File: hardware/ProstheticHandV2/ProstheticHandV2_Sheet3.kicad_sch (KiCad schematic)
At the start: 0 parts

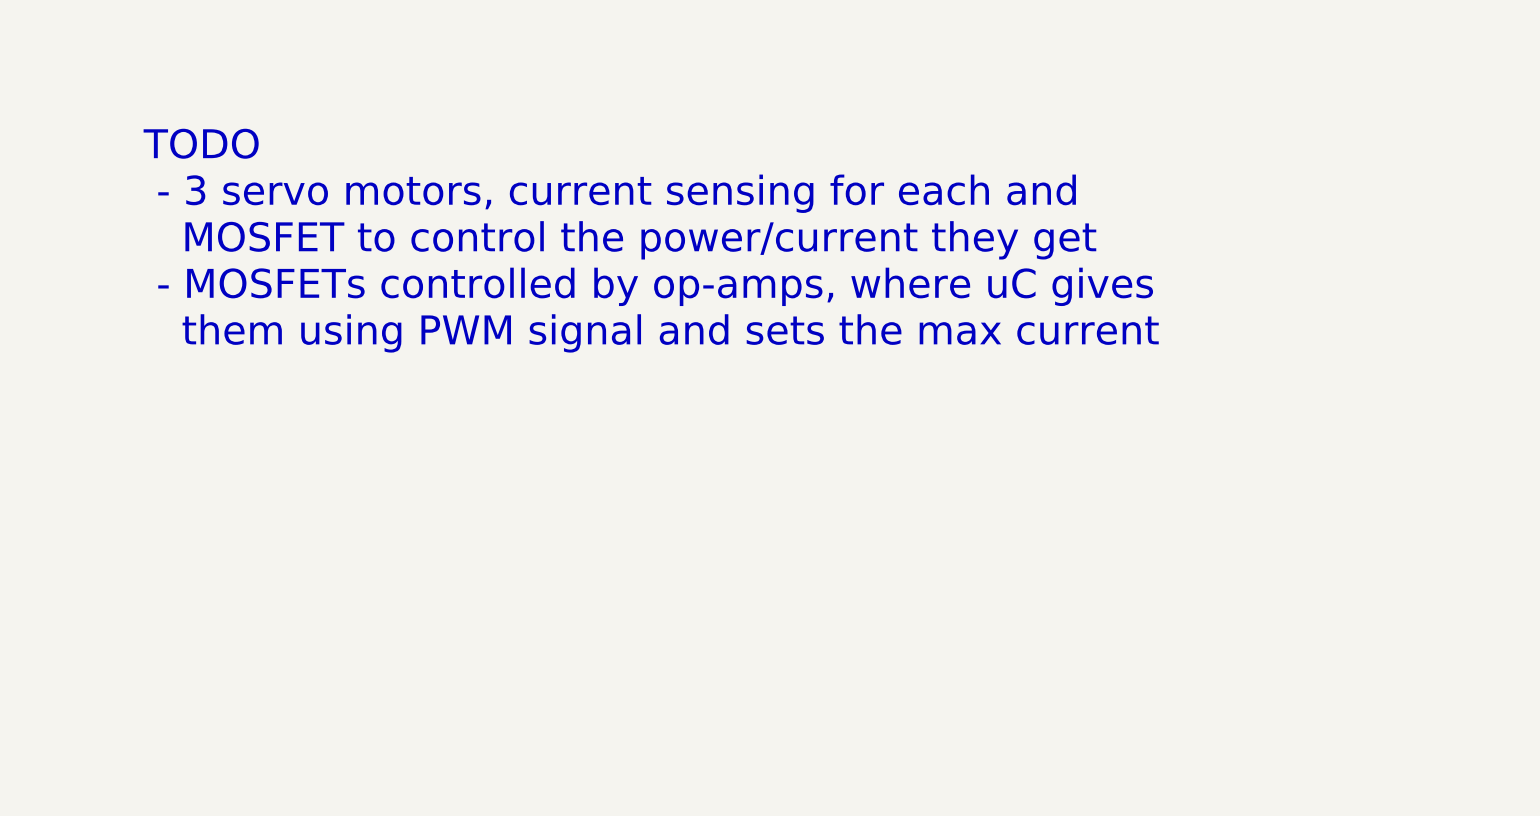
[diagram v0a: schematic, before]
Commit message: Started working on PCB
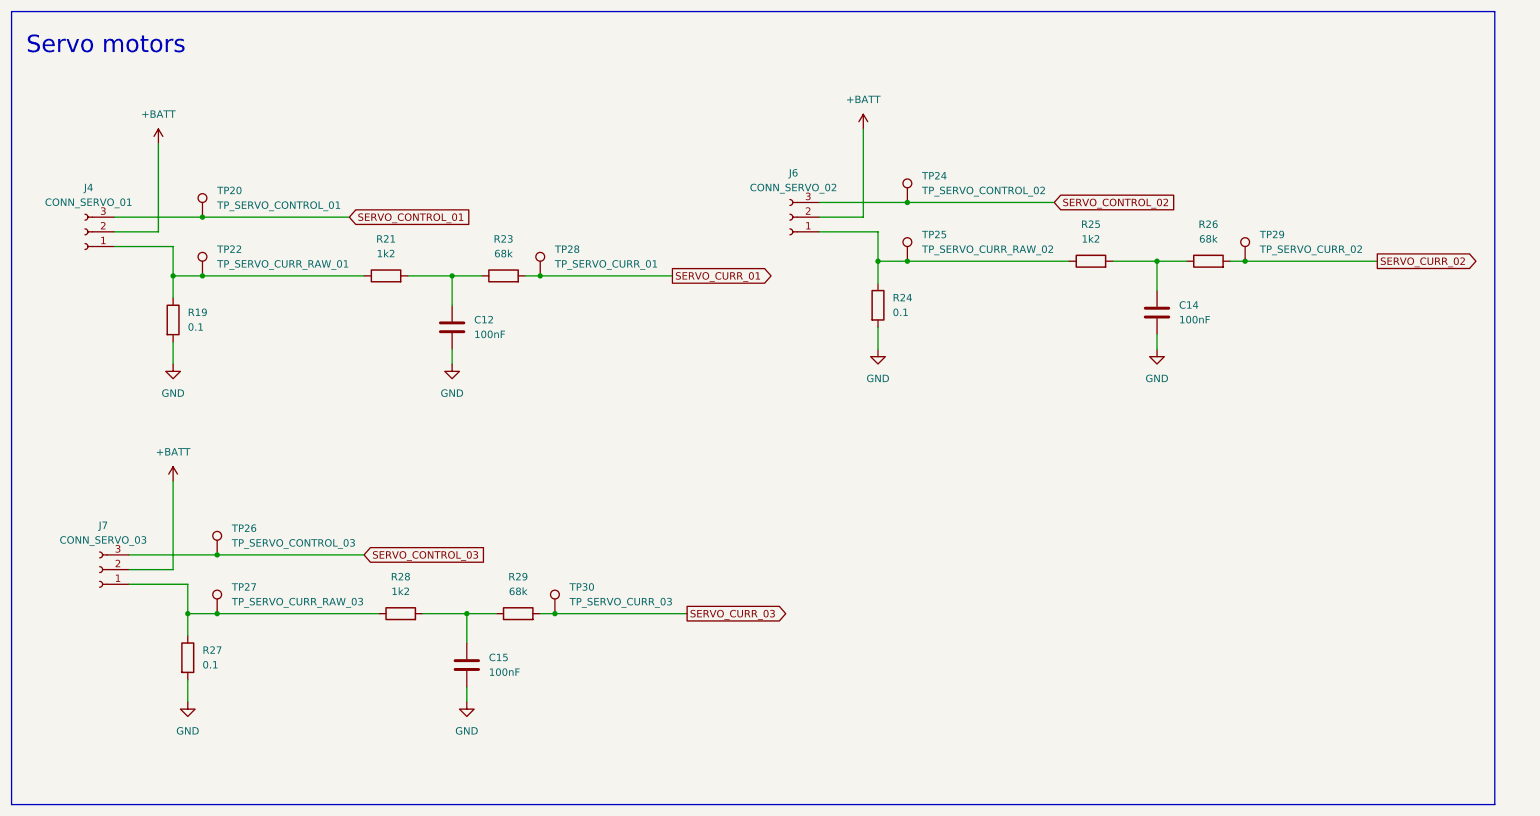
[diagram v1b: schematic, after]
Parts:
- added C12, C14, C15: 100nF, Capacitor_THT:C_Disc_D3.8mm_W2.6mm_P2.50mm, symbol Device:C
- added J4: CONN_SERVO_01, Connector_JST:JST_XA_B03B-XASK-1_1x03_P2.50mm_Vertical, symbol Connector:Conn_01x03_Socket
- added J6: CONN_SERVO_02, Connector_JST:JST_XA_B03B-XASK-1_1x03_P2.50mm_Vertical, symbol Connector:Conn_01x03_Socket
- added J7: CONN_SERVO_03, Connector_JST:JST_XA_B03B-XASK-1_1x03_P2.50mm_Vertical, symbol Connector:Conn_01x03_Socket
- added R19, R24, R27: 0.1, Resistor_THT:R_Axial_DIN0922_L20.0mm_D9.0mm_P30.48mm_Horizontal, symbol Device:R
- added R21, R25, R28: 1k2, Resistor_THT:R_Axial_DIN0207_L6.3mm_D2.5mm_P7.62mm_Horizontal, symbol Device:R
- added R23, R26, R29: 68k, Resistor_THT:R_Axial_DIN0207_L6.3mm_D2.5mm_P7.62mm_Horizontal, symbol Device:R
- added TP20: TP_SERVO_CONTROL_01, TestPoint:TestPoint_Pad_D2.5mm, symbol Connector:TestPoint
- added TP22: TP_SERVO_CURR_RAW_01, TestPoint:TestPoint_Pad_D2.5mm, symbol Connector:TestPoint
- added TP24: TP_SERVO_CONTROL_02, TestPoint:TestPoint_Pad_D2.5mm, symbol Connector:TestPoint
- added TP25: TP_SERVO_CURR_RAW_02, TestPoint:TestPoint_Pad_D2.5mm, symbol Connector:TestPoint
- added TP26: TP_SERVO_CONTROL_03, TestPoint:TestPoint_Pad_D2.5mm, symbol Connector:TestPoint
- added TP27: TP_SERVO_CURR_RAW_03, TestPoint:TestPoint_Pad_D2.5mm, symbol Connector:TestPoint
- added TP28: TP_SERVO_CURR_01, TestPoint:TestPoint_Pad_D2.5mm, symbol Connector:TestPoint
- added TP29: TP_SERVO_CURR_02, TestPoint:TestPoint_Pad_D2.5mm, symbol Connector:TestPoint
- added TP30: TP_SERVO_CURR_03, TestPoint:TestPoint_Pad_D2.5mm, symbol Connector:TestPoint
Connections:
- new net: C14.1, R25.2, R26.1
- new net: J7.1 (Pin_1), R27.1, R28.1, TP27.1
- new net: C15.1, R28.2, R29.1
- new net: J6.1 (Pin_1), R24.1, R25.1, TP25.1
- new net: J4.1 (Pin_1), R19.1, R21.1, TP22.1
- new net: C12.1, R21.2, R23.1
- new net +BATT: J4.2 (Pin_2), J6.2 (Pin_2), J7.2 (Pin_2)
- new net GND: C12.2, C14.2, C15.2, R19.2, R24.2, R27.2
- new net SERVO_CONTROL_01: J4.3 (Pin_3), TP20.1
- new net SERVO_CONTROL_02: J6.3 (Pin_3), TP24.1
- new net SERVO_CONTROL_03: J7.3 (Pin_3), TP26.1
- new net SERVO_CURR_01: R23.2, TP28.1
- new net SERVO_CURR_02: R26.2, TP29.1
- new net SERVO_CURR_03: R29.2, TP30.1
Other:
- note added: "Servo motors"
- note removed: "TODO - 3 servo motors, current sensing for each and MOSFET to control the power/current they get - MOSFETs controlled by op-amps, where uC gives them using PWM signal and sets the max current"
